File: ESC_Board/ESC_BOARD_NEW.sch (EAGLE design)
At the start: 187 parts, among them J3 AVR_SPI_PROG_3X2NS, U2 ATMEGA328P_TQFP, U4 PCA9685

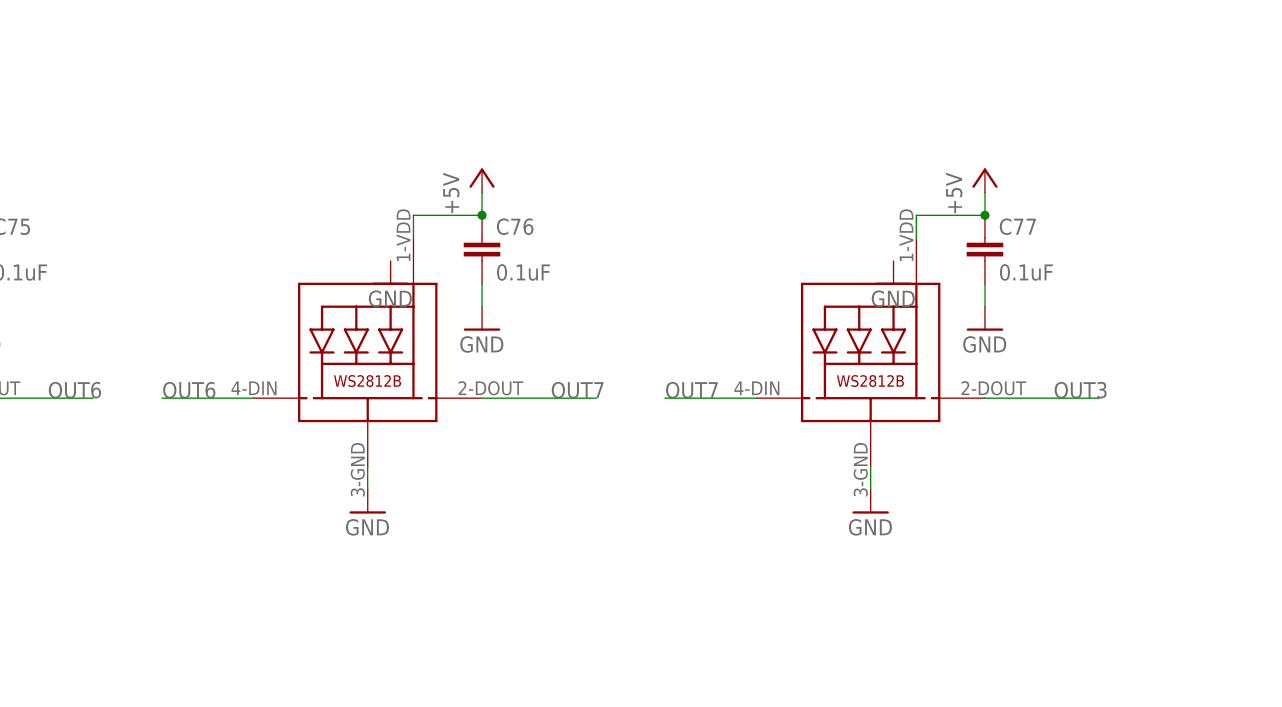
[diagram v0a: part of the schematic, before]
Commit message: More layout stuff
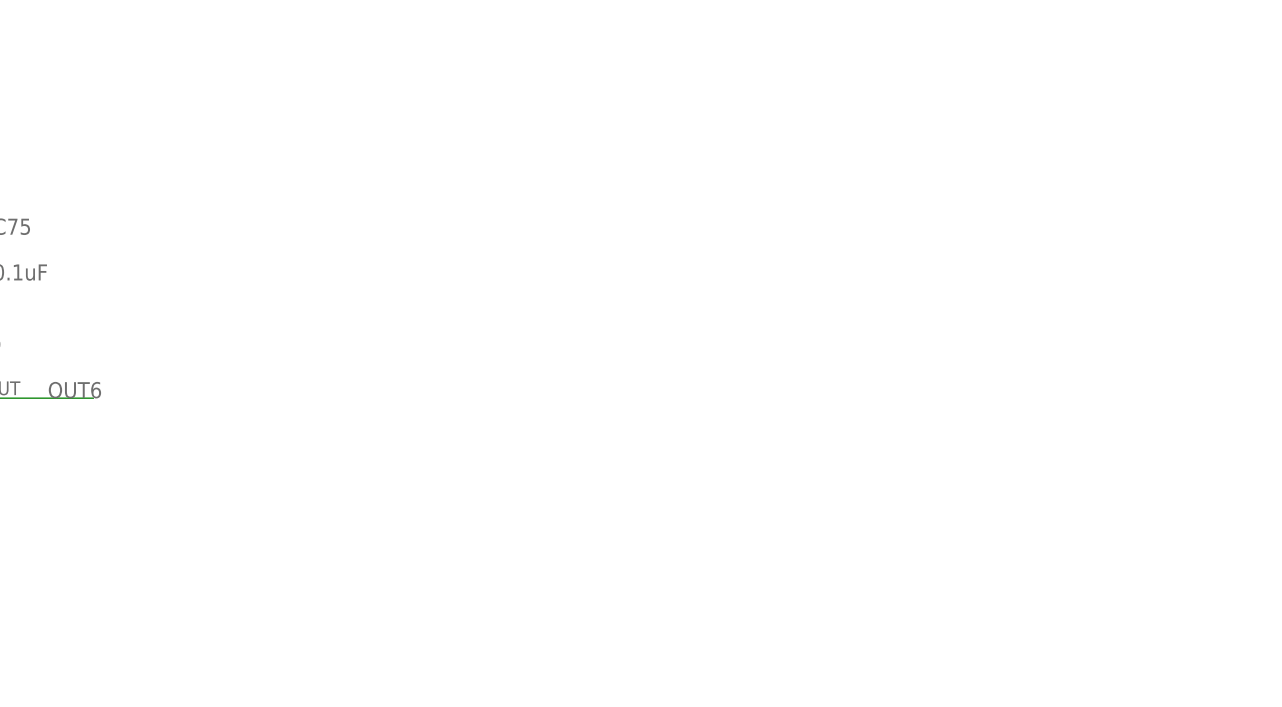
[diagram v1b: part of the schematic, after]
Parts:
- removed C76, C77: 0.1uF, rcl:C-EUC0603
- removed LED7, LED8: WS2812B5050, microbuilder:WS2812B5050
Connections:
- removed net OUT7: LED7.DO, LED8.DI
- net +5V: no longer C76.1, C77.1, LED7.VDD, LED8.VDD
- net GND: no longer C76.2, C77.2, LED7.GND, LED8.GND
- net OUT3: no longer LED8.DO
- net OUT6: no longer LED7.DI
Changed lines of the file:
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@@
 <part name="GND109" library="supply1" library_urn="urn:adsk.eagle:library:371" deviceset="GND" device=""/>
 <part name="GND110" library="supply1" library_urn="urn:adsk.eagle:library:371" deviceset="GND" device=""/>
-<part name="LED7" library="microbuilder" deviceset="WS2812B5050" device="" value="WS2812B5050"/>
-<part name="C76" library="rcl" library_urn="urn:adsk.eagle:library:334" deviceset="C-EU" device="C0603" package3d_urn="urn:adsk.eagle:package:23616/2" value="0.1uF"/>
-<part name="P+41" library="supply1" library_urn="urn:adsk.eagle:library:371" deviceset="+5V" device=""/>
-<part name="GND111" library="supply1" library_urn="urn:adsk.eagle:library:371" deviceset="GND" device=""/>
-<part name="GND112" library="supply1" library_urn="urn:adsk.eagle:library:371" deviceset="GND" device=""/>
-<part name="LED8" library="microbuilder" deviceset="WS2812B5050" device="" value="WS2812B5050"/>
-<part name="C77" library="rcl" library_urn="urn:adsk.eagle:library:334" deviceset="C-EU" device="C0603" package3d_urn="urn:adsk.eagle:package:23616/2" value="0.1uF"/>
-<part name="P+42" library="supply1" library_urn="urn:adsk.eagle:library:371" deviceset="+5V" device=""/>
-<part name="GND113" library="supply1" library_urn="urn:adsk.eagle:library:371" deviceset="GND" device=""/>
-<part name="GND114" library="supply1" library_urn="urn:adsk.eagle:library:371" deviceset="GND" device=""/>
 <part name="P12" library="SparkFun-Connectors" deviceset="M01" device="PTH"/>
 <part name="P13" library="SparkFun-Connectors" deviceset="M01" device="PTH"/>
@@
 <part name="GND116" library="supply1" library_urn="urn:adsk.eagle:library:371" deviceset="GND" device=""/>
 <part name="GND117" library="supply1" library_urn="urn:adsk.eagle:library:371" deviceset="GND" device=""/>
-<part name="GND118" library="supply1" library_urn="urn:adsk.eagle:library:371" deviceset="GND" device=""/>
-<part name="GND119" library="supply1" library_urn="urn:adsk.eagle:library:371" deviceset="GND" device=""/>
 <part name="GND120" library="supply1" library_urn="urn:adsk.eagle:library:371" deviceset="GND" device=""/>
 <part name="GND121" library="supply1" library_urn="urn:adsk.eagle:library:371" deviceset="GND" device=""/>
@@
 <instance part="GND109" gate="1" x="297.18" y="139.7"/>
 <instance part="GND110" gate="1" x="287.02" y="144.78"/>
-<instance part="LED7" gate="G$1" x="340.36" y="134.62"/>
-<instance part="C76" gate="G$1" x="353.06" y="149.86"/>
-<instance part="P+41" gate="1" x="353.06" y="157.48"/>
-<instance part="GND111" gate="1" x="353.06" y="139.7"/>
-<instance part="GND112" gate="1" x="342.9" y="144.78"/>
-<instance part="LED8" gate="G$1" x="396.24" y="134.62"/>
-<instance part="C77" gate="G$1" x="408.94" y="149.86"/>
-<instance part="P+42" gate="1" x="408.94" y="157.48"/>
-<instance part="GND113" gate="1" x="408.94" y="139.7"/>
-<instance part="GND114" gate="1" x="398.78" y="144.78"/>
 <instance part="P12" gate="G$1" x="73.66" y="381" rot="MR0"/>
 <instance part="P13" gate="G$1" x="99.06" y="378.46" rot="MR0"/>
@@
 <instance part="GND116" gate="1" x="340.36" y="180.34"/>
 <instance part="GND117" gate="1" x="396.24" y="180.34"/>
-<instance part="GND118" gate="1" x="396.24" y="119.38"/>
-<instance part="GND119" gate="1" x="340.36" y="119.38"/>
 <instance part="GND120" gate="1" x="284.48" y="119.38"/>
 <instance part="GND121" gate="1" x="228.6" y="119.38"/>
@@
 </segment>
 <segment>
-<pinref part="C76" gate="G$1" pin="2"/>
-<wire x1="353.06" y1="144.78" x2="353.06" y2="142.24" width="0.1524" layer="91"/>
-<pinref part="GND111" gate="1" pin="GND"/>
-</segment>
-<segment>
-<pinref part="C77" gate="G$1" pin="2"/>
-<wire x1="408.94" y1="144.78" x2="408.94" y2="142.24" width="0.1524" layer="91"/>
-<pinref part="GND113" gate="1" pin="GND"/>
-</segment>
-<segment>
 <pinref part="GND121" gate="1" pin="GND"/>
 <pinref part="LED5" gate="G$1" pin="GND"/>
@@
 </segment>
 <segment>
-<pinref part="GND119" gate="1" pin="GND"/>
-<pinref part="LED7" gate="G$1" pin="GND"/>
-<wire x1="340.36" y1="121.92" x2="340.36" y2="124.46" width="0.1524" layer="91"/>
-</segment>
-<segment>
-<pinref part="GND118" gate="1" pin="GND"/>
-<pinref part="LED8" gate="G$1" pin="GND"/>
-<wire x1="396.24" y1="121.92" x2="396.24" y2="124.46" width="0.1524" layer="91"/>
-</segment>
-<segment>
 <pinref part="GND117" gate="1" pin="GND"/>
 <pinref part="LED4" gate="G$1" pin="GND"/>
@@
 <wire x1="297.18" y1="154.94" x2="297.18" y2="152.4" width="0.1524" layer="91"/>
 </segment>
-<segment>
-<pinref part="LED7" gate="G$1" pin="VDD"/>
-<wire x1="345.44" y1="149.86" x2="345.44" y2="152.4" width="0.1524" layer="91"/>
-<pinref part="C76" gate="G$1" pin="1"/>
-<wire x1="345.44" y1="152.4" x2="353.06" y2="152.4" width="0.1524" layer="91"/>
-<junction x="353.06" y="152.4"/>
-<pinref part="P+41" gate="1" pin="+5V"/>
-<wire x1="353.06" y1="154.94" x2="353.06" y2="152.4" width="0.1524" layer="91"/>
-</segment>
-<segment>
-<pinref part="LED8" gate="G$1" pin="VDD"/>
-<wire x1="401.32" y1="149.86" x2="401.32" y2="152.4" width="0.1524" layer="91"/>
-<pinref part="C77" gate="G$1" pin="1"/>
-<wire x1="401.32" y1="152.4" x2="408.94" y2="152.4" width="0.1524" layer="91"/>
-<junction x="408.94" y="152.4"/>
-<pinref part="P+42" gate="1" pin="+5V"/>
-<wire x1="408.94" y1="154.94" x2="408.94" y2="152.4" width="0.1524" layer="91"/>
-</segment>
 </net>
 <net name="N$2" class="0">
@@
 </segment>
 <segment>
-<pinref part="LED8" gate="G$1" pin="DO"/>
-<wire x1="421.64" y1="132.08" x2="408.94" y2="132.08" width="0.1524" layer="91"/>
-<label x="416.56" y="132.08" size="1.778" layer="95"/>
-</segment>
-<segment>
 <pinref part="LED4" gate="G$1" pin="DI"/>
 <wire x1="373.38" y1="195.58" x2="383.54" y2="195.58" width="0.1524" layer="91"/>
@@
 <label x="304.8" y="132.08" size="1.778" layer="95"/>
 </segment>
-<segment>
-<pinref part="LED7" gate="G$1" pin="DI"/>
-<wire x1="317.5" y1="132.08" x2="327.66" y2="132.08" width="0.1524" layer="91"/>
-<label x="317.5" y="132.08" size="1.778" layer="95"/>
-</segment>
-</net>
-<net name="OUT7" class="0">
-<segment>
-<pinref part="LED7" gate="G$1" pin="DO"/>
-<wire x1="365.76" y1="132.08" x2="353.06" y2="132.08" width="0.1524" layer="91"/>
-<label x="360.68" y="132.08" size="1.778" layer="95"/>
-</segment>
-<segment>
-<pinref part="LED8" gate="G$1" pin="DI"/>
-<wire x1="373.38" y1="132.08" x2="383.54" y2="132.08" width="0.1524" layer="91"/>
-<label x="373.38" y="132.08" size="1.778" layer="95"/>
-</segment>
 </net>
